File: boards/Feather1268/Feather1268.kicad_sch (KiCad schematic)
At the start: 32 parts, among them J1 Conn_01x04, J101 Conn_01x03, J102 USB4105-GF-A, J2 Conn_01x04, J3 Conn_01x04, J4 Conn_01x04, J5 Conn_01x04, U101 ESP32-S3-MINI-1U, U102 AMS1117-3.3, U103 ECMF02-2AMX6

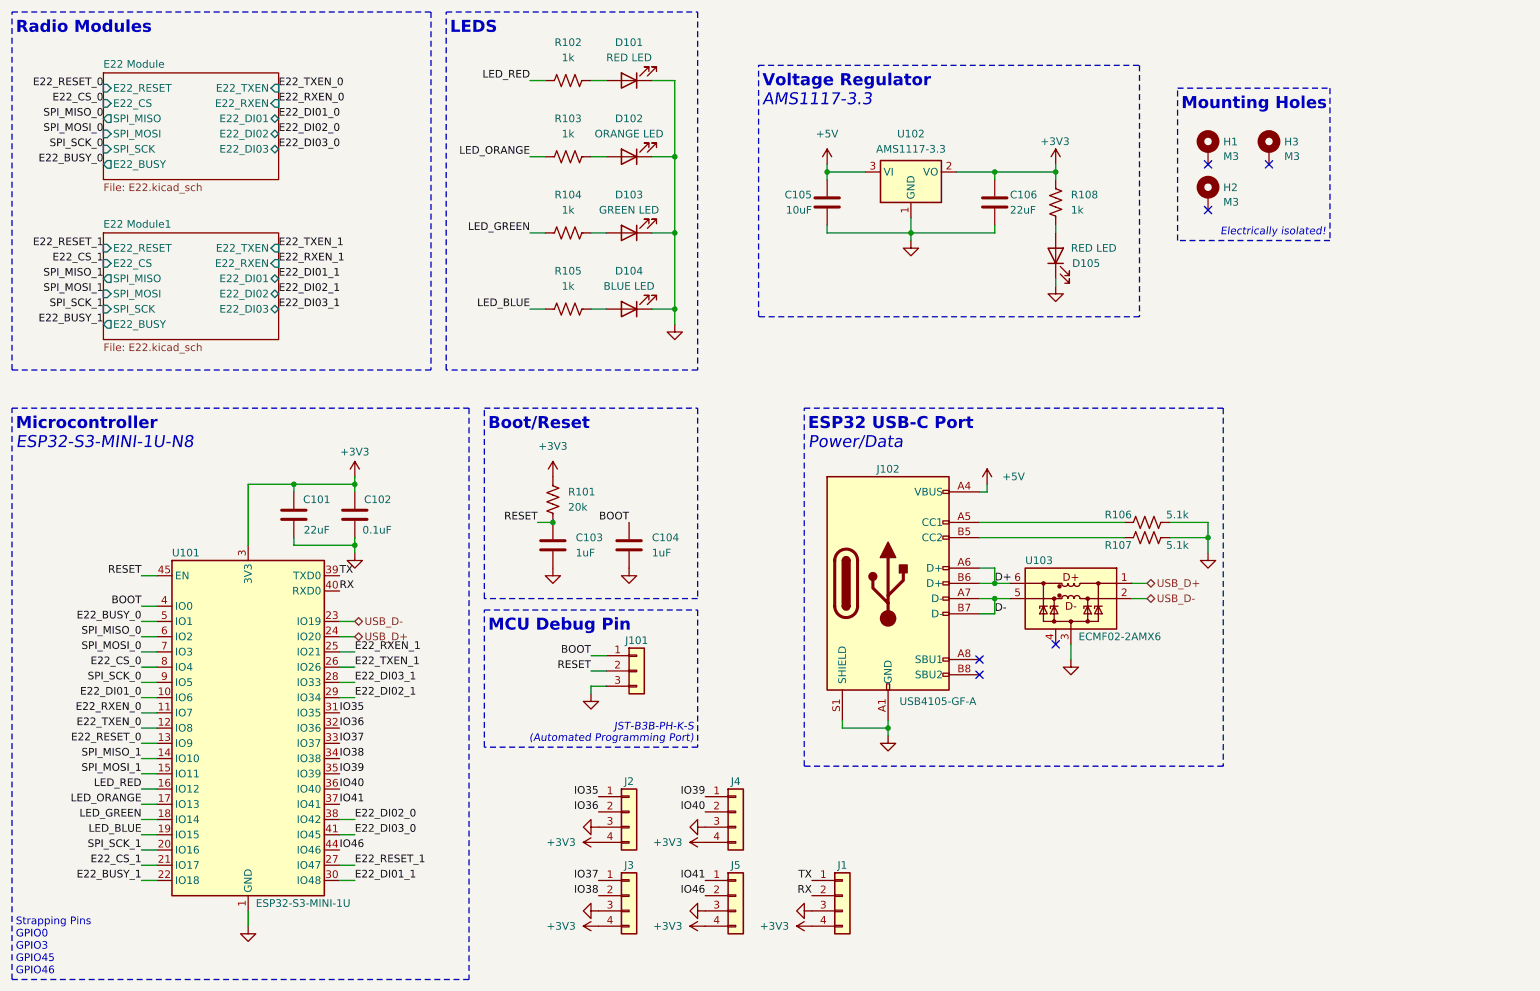
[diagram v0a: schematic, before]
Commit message: minor cleanup
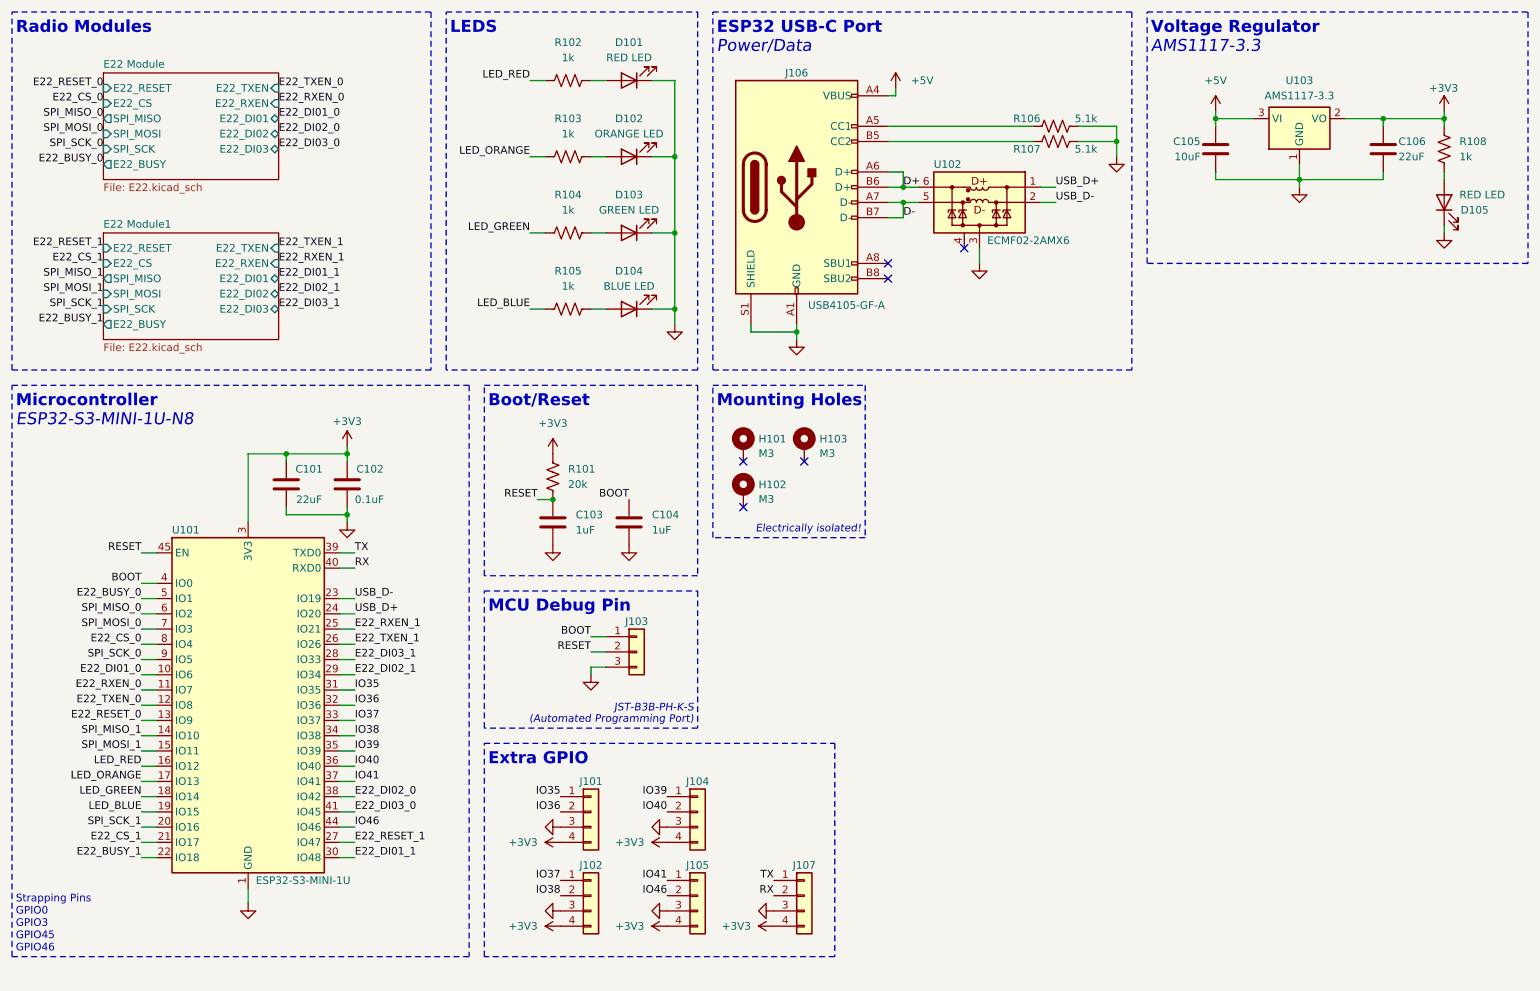
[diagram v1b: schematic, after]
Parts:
- renumbered H1 to H101, H2 to H102, H3 to H103, J2 to J101, J3 to J102, J101 to J103, J4 to J104, J5 to J105, J102 to J106, J1 to J107, U103 to U102, U102 to U103
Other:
- note added: "Extra GPIO"
- moved on the sheet: C101, C102, C103, C104, C105, C106, D105, H101, H102, H103, J101, J102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
